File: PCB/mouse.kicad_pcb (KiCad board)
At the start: 2 copper layers, 3 parts, among them IC1 AH8503-FDC-7, IC2 AH8503-FDC-7, U2 nice_nano

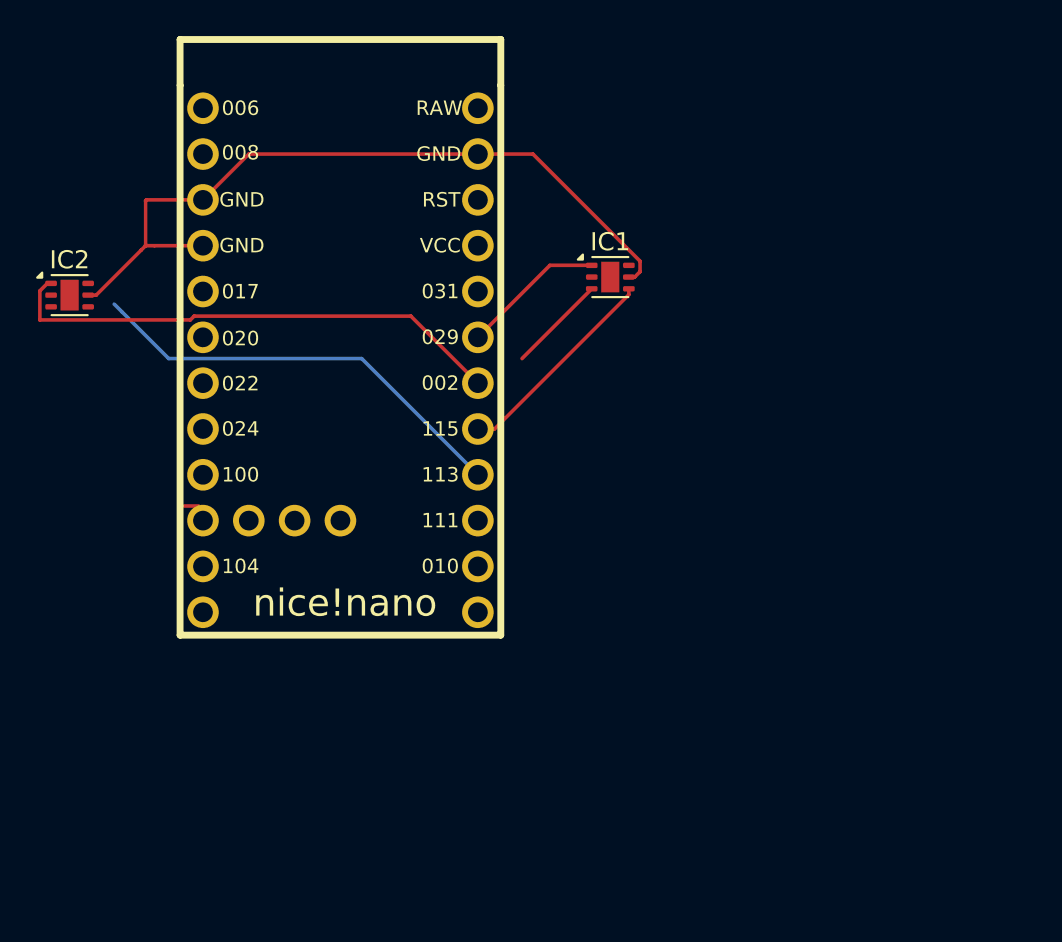
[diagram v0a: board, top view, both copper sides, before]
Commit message: En proceso
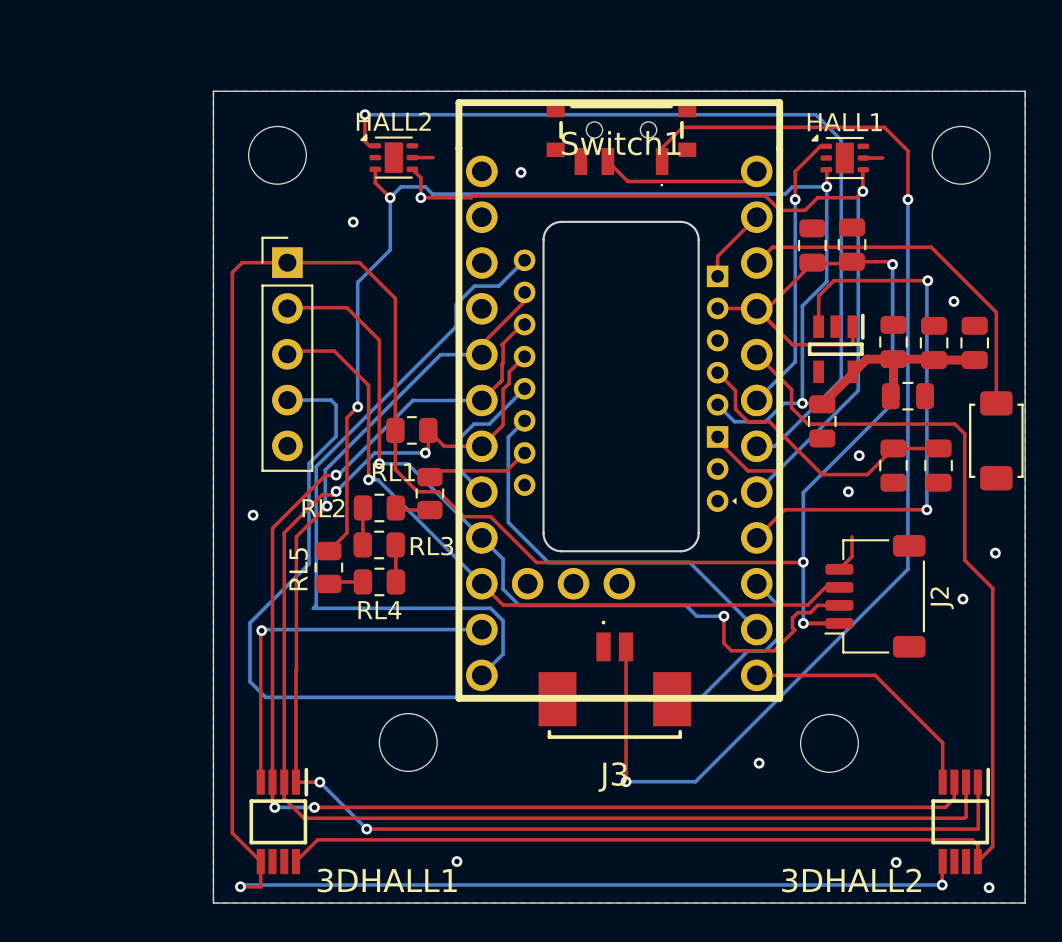
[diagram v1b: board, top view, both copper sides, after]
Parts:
- added 3DHALL1: TMAG5170A2QDGKR, TMAG5170A2QDGKR:SOP65P490X110-8N, F.Cu at (164.6, 118.2)
- added 3DHALL2: TMAG5170A2QDGKR, TMAG5170A2QDGKR:SOP65P490X110-8N, F.Cu at (202.4, 118.2)
- added C1: 4.7uf, Capacitor_SMD:C_0805_2012Metric, F.Cu at (198.7, 98.5)
- added C2: 100nf, Capacitor_SMD:C_0805_2012Metric, F.Cu at (201.2, 98.5)
- added C3: 10uf, Capacitor_SMD:C_0805_2012Metric, F.Cu at (194.2, 86.2)
- added C4: 100nf, Capacitor_SMD:C_0805_2012Metric, F.Cu at (196.4, 86.2)
- added C5: 100nf, Capacitor_SMD:C_0805_2012Metric, F.Cu at (200.9, 91.7)
- added C6: 10uf, Capacitor_SMD:C_0805_2012Metric, F.Cu at (203.2, 91.7)
- added C7: 10uf, Capacitor_SMD:C_0805_2012Metric, F.Cu at (198.7, 91.6)
- added C8: 1uf, Capacitor_SMD:C_0805_2012Metric, F.Cu at (194.8, 96.0)
- added C9: 22uf, Capacitor_SMD:C_0805_2012Metric, F.Cu at (199.5, 94.6)
- added J1: Conn_01x05_Shielded, Connector_PinHeader_2.54mm:PinHeader_1x05_P2.54mm_Vertical, F.Cu at (165.1, 87.2)
- added J2: Conn_01x04_MountingPin, Connector_JST:JST_SH_SM04B-SRSS-TB_1x04-1MP_P1.00mm_Horizontal, F.Cu at (197.7, 105.7)
- added J3: 53261-4002, 53261-4002:532614002, F.Cu at (183.2, 111.0)
- added LDO1.9: TLV70019DDCR, SOT95P280X110-5N:SOT95P280X110-5N, F.Cu at (195.5, 92.0)
- added OpticalSensor1: PAW3395, lib:DIP-16_PAW3395, F.Cu at (183.6, 94.8)
- added R1: 10k, Resistor_SMD:R_0805_2012Metric, F.Cu at (172.0, 96.5)
- added REF**: MountingHole_3.2mm_M3, MountingHole:MountingHole_3.2mm_M3, F.Cu at (202.4, 81.2)
- added REF**: MountingHole_3.2mm_M3, MountingHole:MountingHole_3.2mm_M3, F.Cu at (195.2, 113.8)
- added REF**: MountingHole_3.2mm_M3, MountingHole:MountingHole_3.2mm_M3, F.Cu at (171.8, 113.8)
- added REF**: MountingHole_3.2mm_M3, MountingHole:MountingHole_3.2mm_M3, F.Cu at (164.6, 81.2)
- added RL1: 2.2, Resistor_SMD:R_0805_2012Metric, F.Cu at (173.0, 100.0)
- added RL2: 2.2, Resistor_SMD:R_0805_2012Metric, F.Cu at (170.2, 100.8)
- added RL3: .1, Resistor_SMD:R_0805_2012Metric, F.Cu at (170.2, 102.8)
- added RL4: .1, Resistor_SMD:R_0805_2012Metric, F.Cu at (170.2, 104.9)
- added RL5: 1, Resistor_SMD:R_0805_2012Metric, F.Cu at (167.4, 104.1)
- added SW1: SW_Push, PCM_JLCPCB:SW_TS-1088-AR02016, F.Cu at (204.4, 97.1)
- added Switch1: SSSS811101, SSSS811101:SSSS811101, F.Cu at (183.6, 79.8)
- U2: footprint KiCad:nice_nano -> Nice_nano:nice_nano
- moved HALL2 19.5 mm to (171.0, 81.4)
- moved U2 15.9 mm to (183.5, 96.1)
- moved HALL1 14.6 mm to (196.0, 81.4)
- renumbered IC1 to HALL1, IC2 to HALL2
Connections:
- net 3.3v renamed 1.9v
- HALL1 pad 4: Right_control -> Left_control
- U2 pad 11: unconnected-(U2-P1.04-Pad11) -> CS 2
- U2 pad 12: unconnected-(U2-P1.06-Pad12) -> MOTION
- U2 pad 13: unconnected-(U2-NFC1/P0.09-Pad13) -> CS 3
- U2 pad 14: unconnected-(U2-NFC2/P0.10-Pad14) -> NRESET
- U2 pad 15: unconnected-(U2-P1.11-Pad15) -> INT
- U2 pad 16: Left_control -> EN_LDO
- U2 pad 17: Right_control -> Left_control
- U2 pad 20: unconnected-(U2-AIN7/P0.31-Pad20) -> Alert
- U2 pad 22: unconnected-(U2-RST-Pad22) -> Net-(U2-RST)
- U2 pad 24: unconnected-(U2-BATIN/P0.04-Pad24) -> Interruptor
- U2 pad 8: CS -> CS 1
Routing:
- net +3.3V: track 0.00 -> 167.2 mm, vias 0 -> 5
- net Alert: track 0.00 -> 78.0 mm
- net MOSI: track 0.00 -> 75.4 mm, vias 0 -> 2
- net SCK: track 0.00 -> 75.3 mm, vias 0 -> 3
- net MISO: track 0.00 -> 74.5 mm, vias 0 -> 3
- net 1.9v: track 5.47 -> 79.6 mm, vias 0 -> 4
- net Battery: track 0.00 -> 66.6 mm, vias 0 -> 2
- net INT: track 0.00 -> 54.6 mm
- net SDA: track 0.00 -> 46.0 mm, vias 0 -> 2
- net MOTION: track 0.00 -> 39.3 mm
- net SCL: track 0.81 -> 40.0 mm, vias 0 -> 1
- net EN_LDO: track 0.00 -> 30.9 mm, vias 0 -> 2
- net GND: track 42.3 -> 12.7 mm, vias 0 -> 12
- net Left_control: track 24.1 -> 47.8 mm, vias 0 -> 2
- net NRESET: track 0.00 -> 22.2 mm
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- added copper zone on B.Cu, net GND
- added copper zone on F.Cu, net GND
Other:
- board outline added: 45 x 45 mm
- board text added: "nice!nano"
